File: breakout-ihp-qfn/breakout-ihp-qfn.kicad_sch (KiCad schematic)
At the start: 43 parts, among them J1 Conn_01x12, J2 DF12NB-60DS-0.5V_51, J3 DF12NB-50DS-0.5V_51, U1 AP2112K-1.2, U2 AP2112K-1.8, U3 TT_IHP_ASIC, U4 24LC02

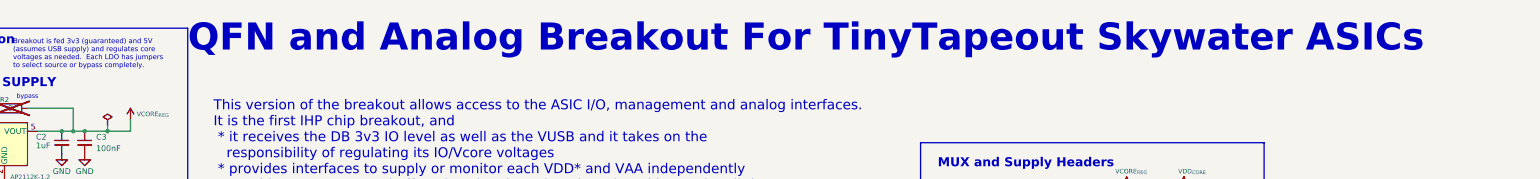
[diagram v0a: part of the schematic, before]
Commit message: IHP schem title tweak
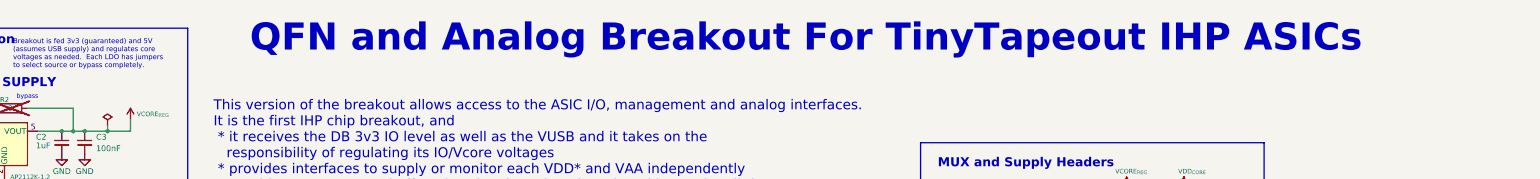
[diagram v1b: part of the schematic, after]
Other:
- note added: "QFN and Analog Breakout For TinyTapeout IHP ASICs"
- note removed: "QFN and Analog Breakout For TinyTapeout Skywater ASICs"
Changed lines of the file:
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@@
 		)
 	)
-	(text "QFN and Analog Breakout For TinyTapeout Skywater ASICs"
+	(text "QFN and Analog Breakout For TinyTapeout IHP ASICs"
 		(exclude_from_sim no)
 		(at 231.14 23.495 0)
